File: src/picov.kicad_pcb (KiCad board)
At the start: 2 copper layers, 21.2 x 51.3 mm, 35 parts, among them J1 USB_C_Receptacle_USB2.0_16P, J2 Conn_01x20, J3 Conn_01x20, J4 Conn_01x03, SW1 Boot, SW2 Reset, SW3 SW_Push, U1 RP2040, U2 AP2112K-3.3, U3 W25Q16JVUXIQ_TR, U4 USBLC6-2SC6, Y1 ABM8-272-T3

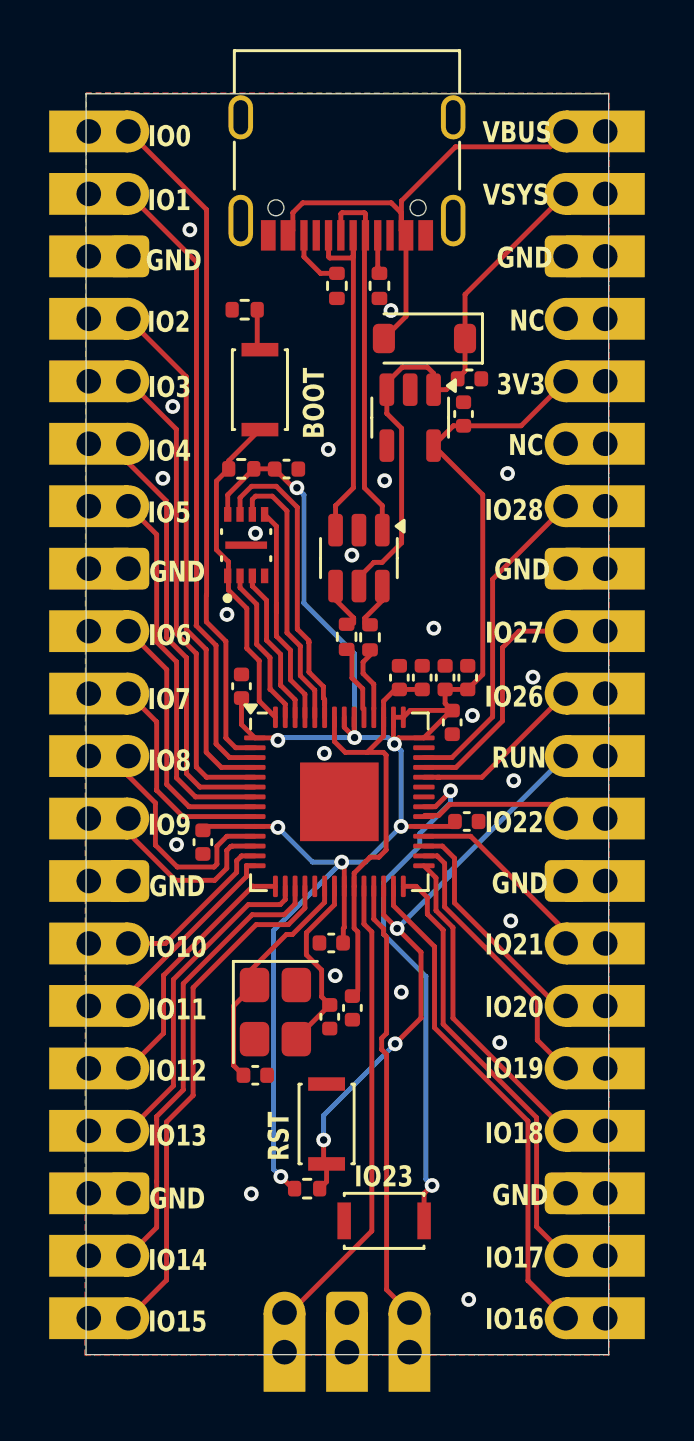
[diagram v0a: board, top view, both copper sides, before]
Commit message: finished pcb!
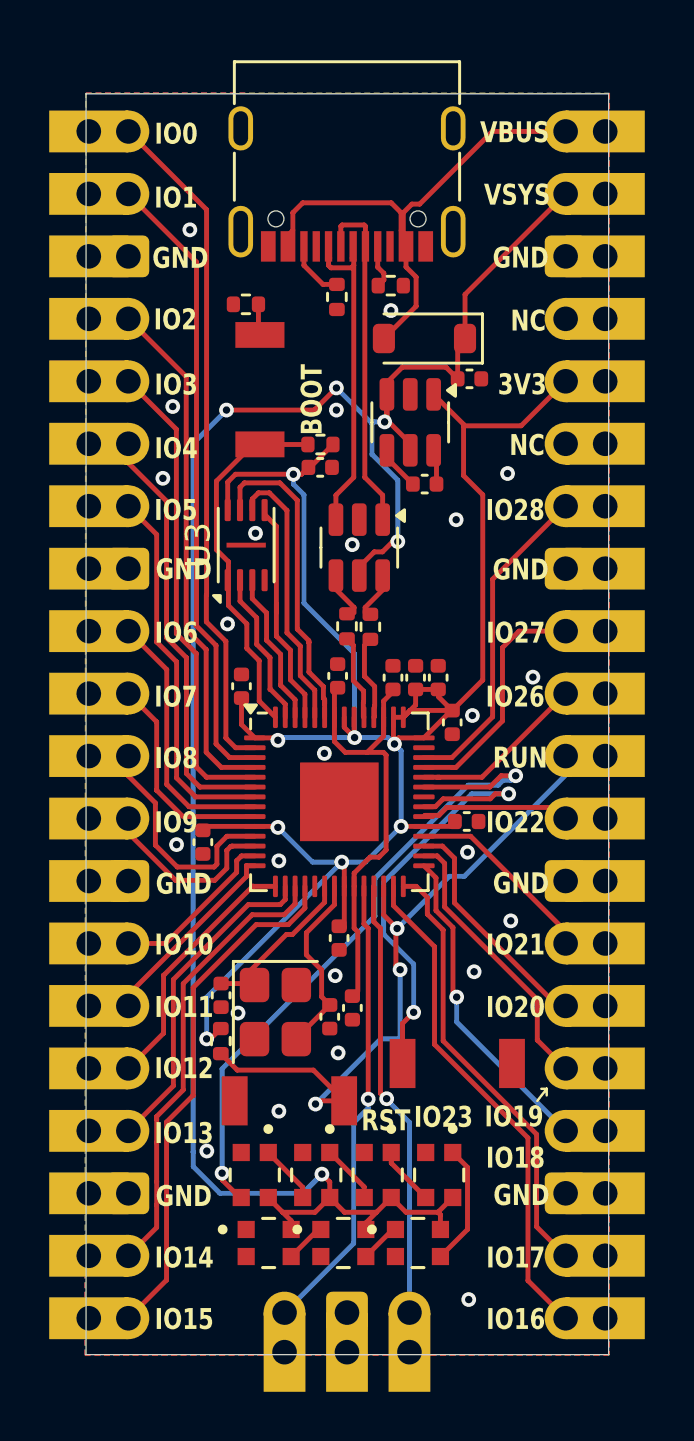
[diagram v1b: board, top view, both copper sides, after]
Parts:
- removed C9: 1uF, Capacitor_SMD:C_0402_1005Metric
- removed U2: AP2112K-3.3, Package_TO_SOT_SMD:SOT-23-5
- added C7: 10uF, Capacitor_SMD:C_0402_1005Metric, F.Cu at (189.3, 59.3)
- added J5: Conn_01x06, Package_TO_SOT_SMD:SOT-23-6, F.Cu at (188.7, 56.8)
- added U10: WS2812-2020, WS2812-2020:LED_WS2812-2020, F.Cu at (186.0, 90.2)
- added U11: WS2812-2020, WS2812-2020:LED_WS2812-2020, F.Cu at (182.9, 90.2)
- added U5: WS2812-2020, WS2812-2020:LED_WS2812-2020, F.Cu at (182.4, 87.4)
- added U6: WS2812-2020, WS2812-2020:LED_WS2812-2020, F.Cu at (184.9, 87.4)
- added U7: WS2812-2020, WS2812-2020:LED_WS2812-2020, F.Cu at (187.4, 87.4)
- added U8: WS2812-2020, WS2812-2020:LED_WS2812-2020, F.Cu at (189.9, 87.4)
- added U9: WS2812-2020, WS2812-2020:LED_WS2812-2020, F.Cu at (189.0, 90.2)
- C1, C12, C13, C2, C3, C4, C5, C6: value 100n -> 100nF
- C10: value 1uF -> 10uF
- C11, C8: value 1u -> 1uF
- R1, R2: value 27.4 -> 27
- SW1: value Boot -> SW_Push; footprint Button_Switch_SMD:SW_SPST_CK_KXT3 -> Button_Switch_SMD:SMD_3x4
- SW2: value Reset -> SW_Push; footprint Button_Switch_SMD:SW_SPST_CK_KXT3 -> Button_Switch_SMD:SMD_3x4
- SW3: footprint Button_Switch_SMD:SW_SPST_CK_KXT3 -> Button_Switch_SMD:SMD_3x4
- U3: footprint W25Q16JVUXIQ_TR:IC_W25Q16JVUXIQ_TR -> Package_SON:Winbond_USON-8-1EP_3x2mm_P0.5mm_EP0.2x1.6mm
- moved SW3 7.06 mm to (190.6, 82.9), turned to 180 degrees
- moved R7 6.95 mm to (181.0, 82.0), turned to -90 degrees
- moved C15 3.53 mm to (181.0, 80.1), turned to 90 degrees
- moved C11 3.44 mm to (185.7, 67.1)
- moved R6 3.37 mm to (185.0, 57.7)
- moved SW2 1.78 mm to (183.8, 84.4), turned to 180 degrees
- moved C14 1.37 mm to (185.0, 58.7)
- moved C2 1.20 mm to (189.8, 67.2)
- moved C8 1.20 mm to (188.9, 67.2)
- moved R3 0.46 mm to (187.9, 51.3), turned to 180 degrees
- moved J1 0.45 mm to (186.1, 46.0)
- moved R4 0.45 mm to (185.7, 51.7)
- moved R1 0.43 mm to (186.1, 65.1)
- moved U4 0.43 mm to (186.6, 61.9)
- moved R2 0.43 mm to (187.1, 65.1)
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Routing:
- net VSYS: track 22.9 -> 82.5 mm, vias 0 -> 5
- net IO25: track 0.00 -> 27.3 mm, vias 0 -> 2
- net Net-(U8-DO): track 0.00 -> 4.93 mm
- net RUN: track 24.6 -> 28.3 mm
- net XIN: track 9.40 -> 6.60 mm
- net IO23: track 20.9 -> 18.3 mm
- net Net-(U7-DO): track 0.00 -> 2.41 mm
- net Net-(U6-DO): track 0.00 -> 2.41 mm
- net Net-(U5-DO): track 0.00 -> 2.41 mm
- net USBDP: track 14.8 -> 13.0 mm
- net Net-(J5-Pin_4): track 0.00 -> 1.81 mm
- net Net-(U10-DI): track 0.00 -> 1.66 mm
- net Net-(U10-DO): track 0.00 -> 1.66 mm
- net SPI_CS: track 13.4 -> 14.9 mm
- net Net-(J5-Pin_6): track 0.00 -> 1.42 mm
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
